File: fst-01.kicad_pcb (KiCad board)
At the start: 2 copper layers, 21 x 12.6 mm, 19 parts, among them J1 USB_A, K1 CONN_3, U1 STM32F103TB, U2 MCP1700-3302E, U3 NUF2221W1, U5 X2SON, X1 12MHz

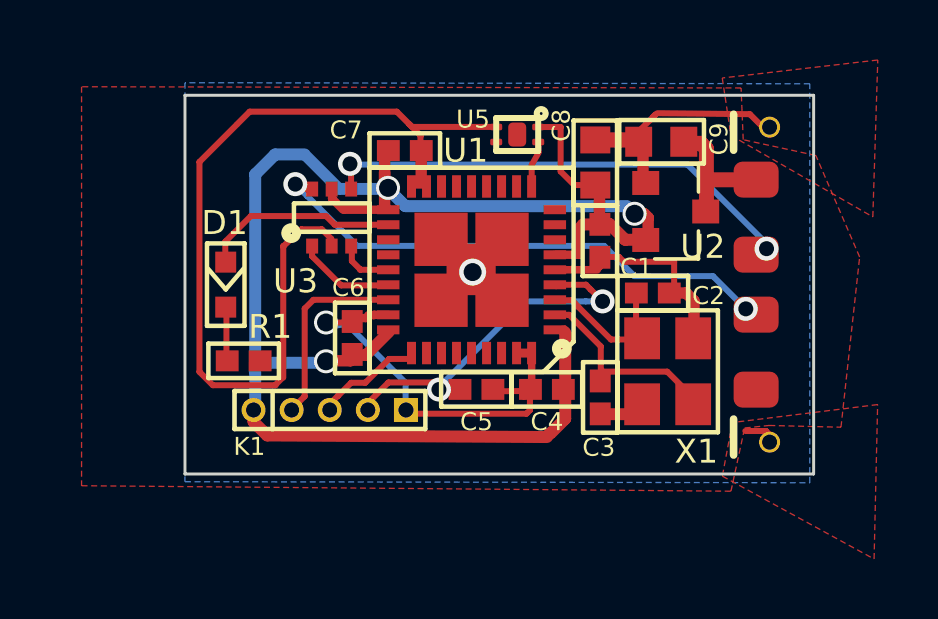
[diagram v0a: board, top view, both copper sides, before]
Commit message: More change to PCBA.
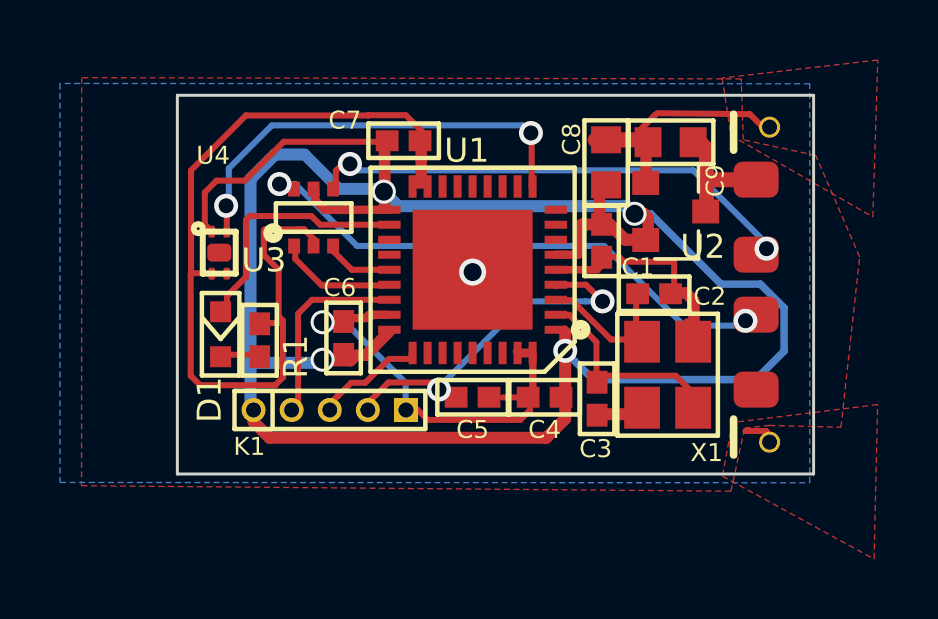
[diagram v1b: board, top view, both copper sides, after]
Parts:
- moved U4 10.7 mm to (109.9, 97.9), turned to 0 degrees
- moved D1 1.66 mm to (109.9, 100.7)
- moved R1 0.87 mm to (111.2, 100.8), turned to 270 degrees
- moved U3 0.60 mm to (113.0, 96.8)
- moved C8 0.36 mm to (122.8, 94.9)
- moved C7 0.33 mm to (116.0, 94.2)
- moved C9 0.31 mm to (124.9, 94.2)
- moved C5 0.29 mm to (118.3, 102.8)
- moved C6 0.29 mm to (114.0, 100.8)
- moved C4 0.27 mm to (120.7, 102.8)
- moved X1 0.11 mm to (124.8, 102.0)
- moved C3 0.11 mm to (122.5, 102.8)
- moved C1 0.06 mm to (122.6, 97.5)
- renumbered U5 to U4
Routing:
- net +3V3: track 56.1 -> 77.0 mm, vias 3 -> 4
- net /PA3: track 1.49 -> 14.7 mm, vias 0 -> 2
- net GND: track 80.8 -> 73.3 mm
- net /LED: track 6.59 -> 8.28 mm
- net /D+_PLUG: track 17.4 -> 18.1 mm
- net /D+: track 3.30 -> 3.94 mm
- net /VBUS: track 4.36 -> 3.80 mm
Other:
- board size 21 x 12.6 mm -> 21.2 x 12.6 mm
